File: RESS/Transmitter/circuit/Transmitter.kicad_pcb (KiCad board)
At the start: 2 copper layers, 42 x 45 mm, 17 parts, among them J3 ADP_L, J4 ADP_R, J5 POWER, J6 ESS_IN, SW1 SW_SPDT, U1 BP5293

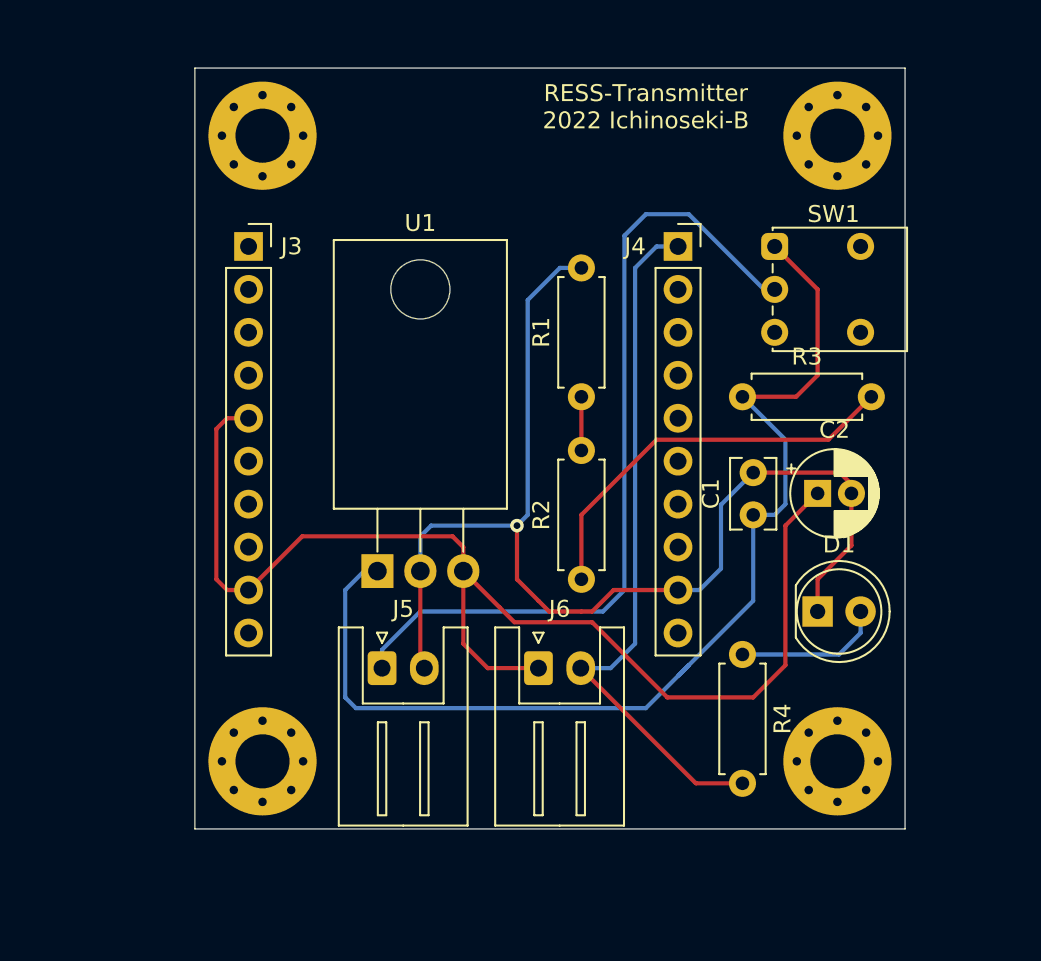
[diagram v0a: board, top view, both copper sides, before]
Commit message: WIP
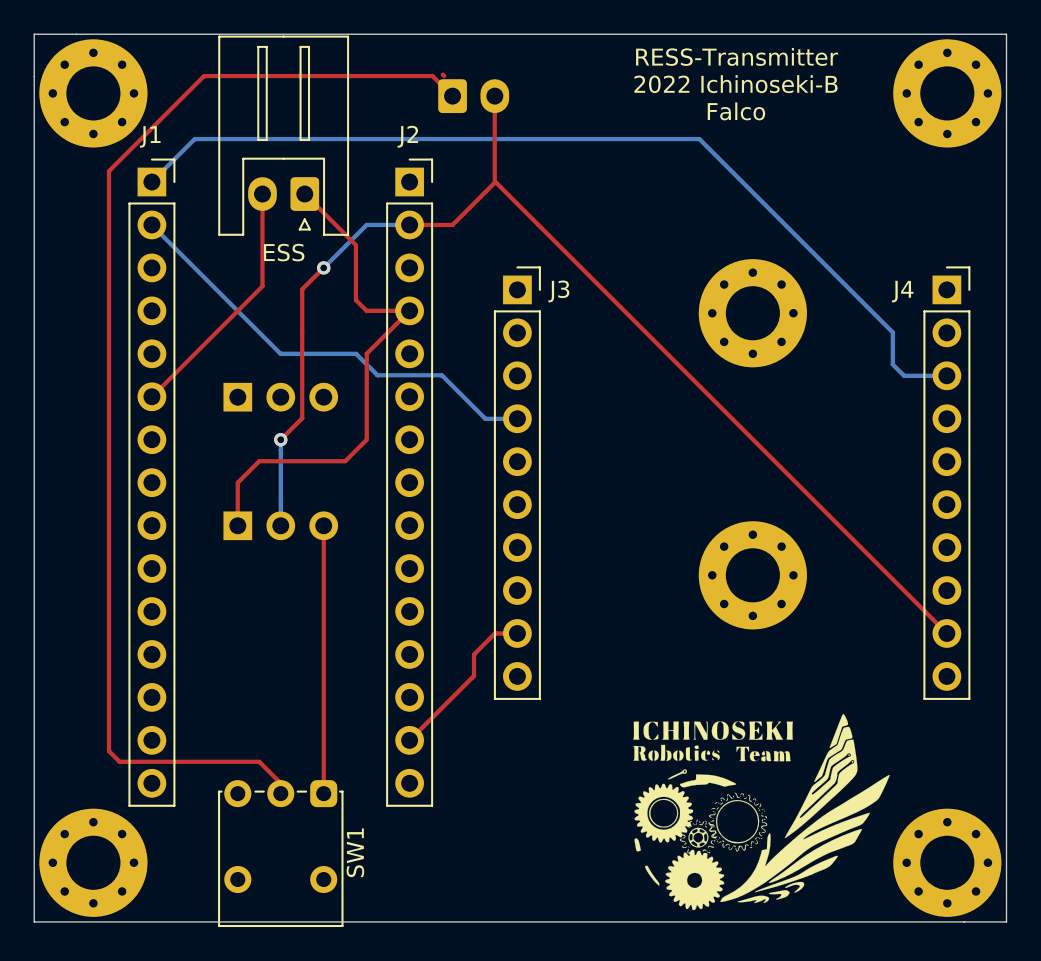
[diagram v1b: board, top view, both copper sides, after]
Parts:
- removed C1: 0.33μF, Capacitor_THT:C_Rect_L4.0mm_W2.5mm_P2.50mm
- removed C2: 47μF, Capacitor_THT:CP_Radial_D5.0mm_P2.00mm
- removed D1: LED, LED_THT:LED_D5.0mm
- removed H1, H2, H3, H4: MountingHole, MountingHole:MountingHole_3.2mm_M3_Pad_Via
- removed J6: ESS_IN, Connector_JST:JST_XH_S2B-XH-A_1x02_P2.50mm_Horizontal
- removed R1, R2, R3: 22Ω, Resistor_THT:R_Axial_DIN0207_L6.3mm_D2.5mm_P7.62mm_Horizontal
- removed R4: 330Ω, Resistor_THT:R_Axial_DIN0207_L6.3mm_D2.5mm_P7.62mm_Horizontal
- removed U1: BP5293, Package_TO_SOT_THT:TO-220-3_Horizontal_TabDown
- added ESS: ESS_IN, Connector_JST:JST_XH_S2B-XH-A_1x02_P2.50mm_Horizontal, F.Cu at (133.5, 79.5)
- added J1: Conn_01x15_Female, Connector_PinSocket_2.54mm:PinSocket_1x15_P2.54mm_Vertical, F.Cu at (124.5, 78.7)
- added J2: Conn_01x15_Female, Connector_PinSocket_2.54mm:PinSocket_1x15_P2.54mm_Vertical, F.Cu at (139.7, 78.7)
- added J7: Conn_01x03_Female, Connector_PinSocket_2.54mm:PinSocket_1x03_P2.54mm_Vertical, B.Cu at (129.5, 91.5)
- added J8: Logo, INCT:INCT, F.Cu at (159.8, 115.2)
- added J8: Conn_01x03_Female, Connector_PinSocket_2.54mm:PinSocket_1x03_P2.54mm_Vertical, B.Cu at (129.5, 99.1)
- added REF**: MountingHole_3.2mm_M3_Pad_Via, MountingHole:MountingHole_3.2mm_M3_Pad_Via, F.Cu at (121.0, 119.0)
- added REF**: MountingHole_3.2mm_M3_Pad_Via, MountingHole:MountingHole_3.2mm_M3_Pad_Via, F.Cu at (171.5, 119.0)
- added REF**: MountingHole_3.2mm_M3_Pad_Via, MountingHole:MountingHole_3.2mm_M3_Pad_Via, F.Cu at (121.0, 73.5)
- added REF**: MountingHole_3.2mm_M3_Pad_Via, MountingHole:MountingHole_3.2mm_M3_Pad_Via, F.Cu at (160.0, 86.5)
- added REF**: MountingHole_3.2mm_M3_Pad_Via, MountingHole:MountingHole_3.2mm_M3_Pad_Via, F.Cu at (160.0, 102.0)
- added REF**: MountingHole_3.2mm_M3_Pad_Via, MountingHole:MountingHole_3.2mm_M3_Pad_Via, F.Cu at (171.5, 73.5)
- J5: footprint Connector_JST:JST_XH_S2B-XH-A_1x02_P2.50mm_Horizontal -> Connector_JST:JST_XH_B2B-XH-A_1x02_P2.50mm_Vertical; moved to B.Cu
- moved SW1 41.9 mm to (134.6, 114.9), turned to -90 degrees
- moved J5 34.1 mm to (142.2, 73.7)
- moved J4 16.1 mm to (171.5, 85.1)
- moved J3 16.1 mm to (146.1, 85.1)
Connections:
- J3 pad 1: (no net) -> Net-(J3-Pad1)
- J3 pad 10: (no net) -> Net-(J3-Pad10)
- J3 pad 2: (no net) -> Net-(J3-Pad2)
- J3 pad 3: (no net) -> Net-(J3-Pad3)
- J3 pad 4: (no net) -> RX
- J3 pad 5: +3V3 -> Net-(J3-Pad5)
- J3 pad 6: (no net) -> Net-(J3-Pad6)
- J3 pad 7: (no net) -> Net-(J3-Pad7)
- J3 pad 8: (no net) -> Net-(J3-Pad8)
- J4 pad 1: ESS -> Net-(J4-Pad1)
- J4 pad 10: (no net) -> Net-(J4-Pad10)
- J4 pad 2: (no net) -> Net-(J4-Pad2)
- J4 pad 3: (no net) -> TX
- J4 pad 4: (no net) -> Net-(J4-Pad4)
- J4 pad 5: (no net) -> Net-(J4-Pad5)
- J4 pad 6: (no net) -> Net-(J4-Pad6)
- J4 pad 7: (no net) -> Net-(J4-Pad7)
- J4 pad 8: (no net) -> Net-(J4-Pad8)
- SW1 pad 1: +5V -> VCC
- SW1 pad 3: (no net) -> Net-(SW1-Pad3)
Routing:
- net +3V3: track 72.1 -> 9.76 mm
- net TX: track 0.00 -> 55.0 mm
- net ESS: track 41.5 -> 0.00 mm
- net +5V: track 64.9 -> 30.9 mm
- net RX: track 0.00 -> 26.4 mm
- net Net-(R2-Pad1): track 23.8 -> 0.00 mm
- net PW_IN: track 49.1 -> 69.1 mm
- net VCC: track 0.00 -> 15.8 mm
- net ESS_IN: track 0.00 -> 14.7 mm
- net LED: track 8.78 -> 0.00 mm
- net Net-(R1-Pad1): track 3.17 -> 0.00 mm
- net GND: track 69.4 -> 71.4 mm, vias 1 -> 2
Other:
- board size 42 x 45 mm -> 57.5 x 52.5 mm
- net class Default removed
- board text added: "JLCJLCJLC"
- board text added: "RESS-Transmitter 2022 Ichinoseki-B Falco"
- board text removed: "JLCJLCJLCJLC"
- board text removed: "RESS-Transmitter 2022 Ichinoseki-B"
